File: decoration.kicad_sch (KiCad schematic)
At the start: 9 parts, among them J12 Fuse holder or smth to hold t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

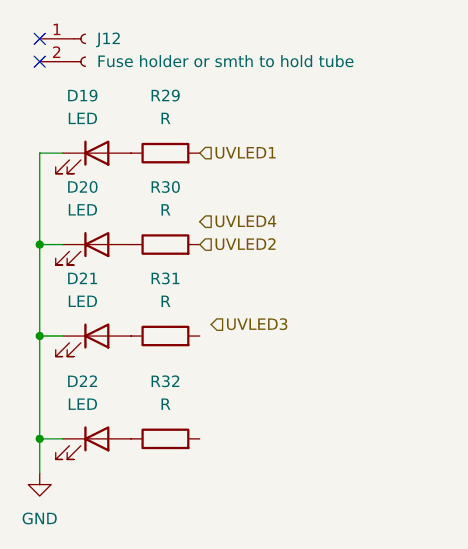
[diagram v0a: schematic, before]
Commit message: Autosave
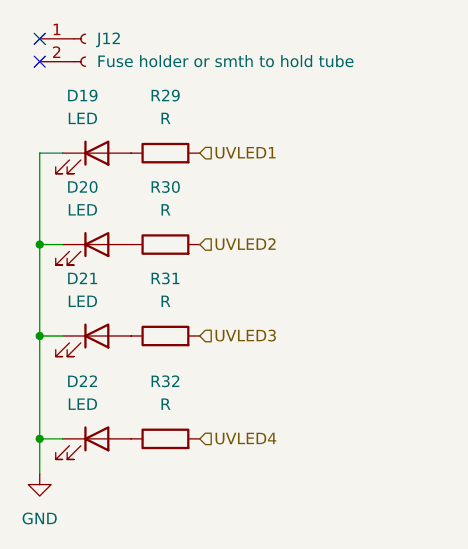
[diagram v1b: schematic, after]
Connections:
- net UVLED3: now also R31.2
- net UVLED4: now also R32.2
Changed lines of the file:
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@@
 	(hierarchical_label "UVLED4"
 		(shape input)
-		(at 123.19 85.09 0)
+		(at 123.19 109.22 0)
 		(effects
 			(font
@@
 	(hierarchical_label "UVLED3"
 		(shape input)
-		(at 124.46 96.52 0)
+		(at 123.19 97.79 0)
 		(effects
 			(font
